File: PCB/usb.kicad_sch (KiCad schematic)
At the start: 52 parts, among them J2 Conn_ARM_SWD_TagConnect_TC2030, J4 TYPE-C-31-M-12, U10 FT2232HQ, U3 TPD2EUSB30, U4 TPD2EUSB30, U6 TPD2EUSB30, U8 TPS62132, U9 M93C56-WMN6TP, Y2 12MHz

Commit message: buttons, more footprints, some other stuff
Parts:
- R29, R32, R36, R37: footprint (none) -> Resistor_SMD:R_0402_1005Metric
- Y2: footprint (none) -> Crystal:Crystal_SMD_3225-4Pin_3.2x2.5mm
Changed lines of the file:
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@@
 			)
 		)
-		(property "Footprint" ""
+		(property "Footprint" "Crystal:Crystal_SMD_3225-4Pin_3.2x2.5mm"
 			(at 125.73 243.84 0)
 			(effects
@@
 			)
 		)
-		(property "Footprint" ""
+		(property "Footprint" "Resistor_SMD:R_0402_1005Metric"
 			(at 293.37 166.878 90)
 			(effects
@@
 			)
 		)
-		(property "Footprint" ""
+		(property "Footprint" "Resistor_SMD:R_0402_1005Metric"
 			(at 293.37 169.418 90)
 			(effects
@@
 			)
 		)
-		(property "Footprint" ""
+		(property "Footprint" "Resistor_SMD:R_0402_1005Metric"
 			(at 293.37 161.798 90)
 			(effects
@@
 			)
 		)
-		(property "Footprint" ""
+		(property "Footprint" "Resistor_SMD:R_0402_1005Metric"
 			(at 293.37 164.338 90)
 			(effects

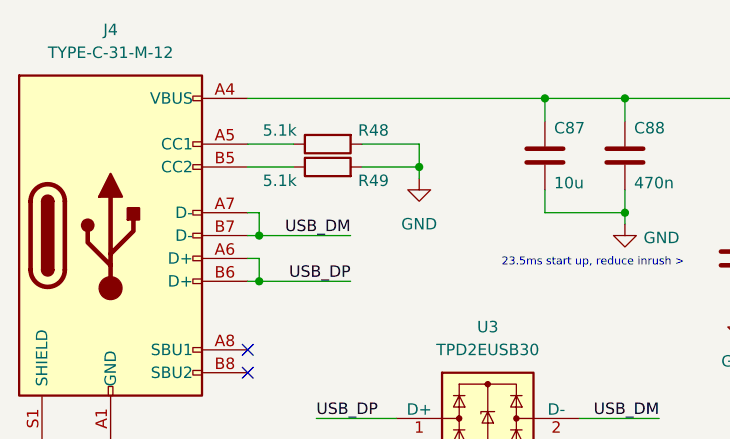
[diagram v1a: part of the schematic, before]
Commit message: adding most of the resistor footprints
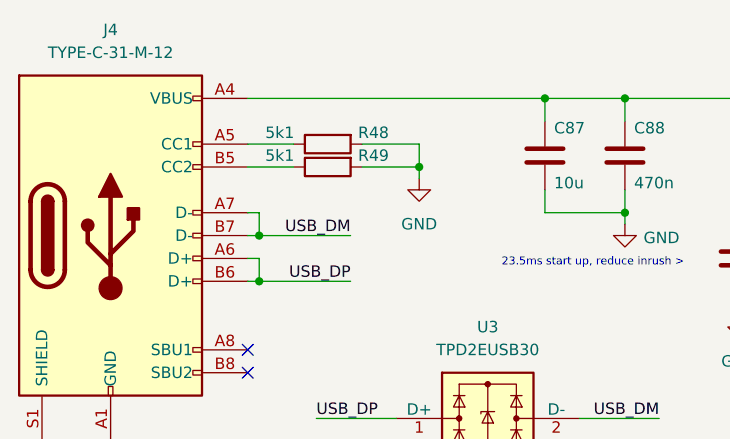
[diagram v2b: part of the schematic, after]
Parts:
- R38, R39, R40, R41, R51, R53, R54: footprint (none) -> Resistor_SMD:R_0402_1005Metric
- R48, R49: value 5.1k -> 5k1
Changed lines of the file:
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@@
 			)
 		)
-		(property "Footprint" ""
+		(property "Footprint" "Resistor_SMD:R_0402_1005Metric"
 			(at 94.742 217.17 90)
 			(effects
@@
 	)
 	(symbol
+		(lib_id "Device:R")
+		(at 59.69 35.56 90)
+		(mirror x)
+		(unit 1)
+		(exclude_from_sim no)
+		(in_bom yes)
+		(on_board yes)
+		(dnp no)
+		(property "Reference" "R49"
+			(at 64.77 34.29 90)
+			(effects
+				(font
+					(size 1.27 1.27)
+				)
+			)
+		)
+		(property "Value" "5k1"
+			(at 54.356 34.29 90)
+			(effects
+				(font
+					(size 1.27 1.27)
+				)
+			)
+		)
+		(property "Footprint" ""
+			(at 59.69 33.782 90)
+			(effects
+				(font
+					(size 1.27 1.27)
+				)
+				(hide yes)
+			)
+		)
+		(property "Datasheet" "~"
+			(at 59.69 35.56 0)
+			(effects
+				(font
+					(size 1.27 1.27)
+				)
+				(hide yes)
+			)
+		)
+		(property "Description" "Resistor"
+			(at 59.69 35.56 0)
+			(effects
+				(font
+					(size 1.27 1.27)
+				)
+				(hide yes)
+			)
+		)
+		(pin "2"
+		)
+		(pin "1"
+		)
+		(instances
+			(project "PCB"
+				(path "/ed0095eb-57a0-4856-9ac4-7b40bd214a3a/b3feae67-f5ac-44a3-90a4-88fd0a4da47c"
+					(reference "R49")
+					(unit 1)
+				)
+			)
+		)
+	)
+	(symbol
 		(lib_id "Device:C")
 		(at 119.38 170.18 0)
@@
 			)
 		)
-		(property "Footprint" ""
+		(property "Footprint" "Resistor_SMD:R_0402_1005Metric"
 			(at 304.292 151.13 90)
 			(effects
@@
 	)
 	(symbol
-		(lib_id "Device:R")
-		(at 59.69 35.56 90)
-		(unit 1)
-		(exclude_from_sim no)
-		(in_bom yes)
-		(on_board yes)
-		(dnp no)
-		(property "Reference" "R49"
-			(at 64.77 37.084 90)
-			(effects
-				(font
-					(size 1.27 1.27)
-				)
-			)
-		)
-		(property "Value" "5.1k"
-			(at 54.356 37.084 90)
-			(effects
-				(font
-					(size 1.27 1.27)
-				)
-			)
-		)
-		(property "Footprint" ""
-			(at 59.69 37.338 90)
-			(effects
-				(font
-					(size 1.27 1.27)
-				)
-				(hide yes)
-			)
-		)
-		(property "Datasheet" "~"
-			(at 59.69 35.56 0)
-			(effects
-				(font
-					(size 1.27 1.27)
-				)
-				(hide yes)
-			)
-		)
-		(property "Description" "Resistor"
-			(at 59.69 35.56 0)
-			(effects
-				(font
-					(size 1.27 1.27)
-				)
-				(hide yes)
-			)
-		)
-		(pin "2"
-		)
-		(pin "1"
-		)
-		(instances
-			(project "PCB"
-				(path "/ed0095eb-57a0-4856-9ac4-7b40bd214a3a/b3feae67-f5ac-44a3-90a4-88fd0a4da47c"
-					(reference "R49")
-					(unit 1)
-				)
-			)
-		)
-	)
-	(symbol
 		(lib_id "Power_Protection:TPD2EUSB30")
 		(at 261.62 204.47 0)
@@
 			)
 		)
-		(property "Footprint" ""
+		(property "Footprint" "Resistor_SMD:R_0402_1005Metric"
 			(at 330.962 151.13 90)
 			(effects
@@
 			)
 		)
-		(property "Footprint" ""
+		(property "Footprint" "Resistor_SMD:R_0402_1005Metric"
 			(at 76.962 217.17 90)
 			(effects
@@
 			)
 		)
-		(property "Footprint" ""
+		(property "Footprint" "Resistor_SMD:R_0402_1005Metric"
 			(at 322.072 151.13 90)
 			(effects
@@
 		(dnp no)
 		(property "Reference" "R48"
-			(at 64.77 31.496 90)
+			(at 64.77 31.75 90)
 			(effects
 				(font
@@
 			)
 		)
-		(property "Value" "5.1k"
-			(at 54.356 31.496 90)
+		(property "Value" "5k1"
+			(at 54.356 31.75 90)
 			(effects
 				(font
@@
 			)
 		)
-		(property "Footprint" ""
+		(property "Footprint" "Resistor_SMD:R_0402_1005Metric"
 			(at 85.852 217.17 90)
 			(effects
@@
 			)
 		)
-		(property "Footprint" ""
+		(property "Footprint" "Resistor_SMD:R_0402_1005Metric"
 			(at 313.182 151.13 90)
 			(effects

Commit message: finisehed upassigning resistor footprints
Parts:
- C89: footprint (none) -> Capacitor_SMD:C_0603_1608Metric
- R48, R49, R50, R52, R55, R56, R76: footprint (none) -> Resistor_SMD:R_0402_1005Metric
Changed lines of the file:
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@@
 			)
 		)
-		(property "Footprint" ""
+		(property "Footprint" "Capacitor_SMD:C_0603_1608Metric"
 			(at 106.3752 49.53 0)
 			(effects
@@
 			)
 		)
-		(property "Footprint" ""
+		(property "Footprint" "Resistor_SMD:R_0402_1005Metric"
 			(at 59.69 33.782 90)
 			(effects
@@
 			)
 		)
-		(property "Footprint" ""
+		(property "Footprint" "Resistor_SMD:R_0402_1005Metric"
 			(at 130.81 199.898 90)
 			(effects
@@
 			)
 		)
-		(property "Footprint" ""
+		(property "Footprint" "Resistor_SMD:R_0402_1005Metric"
 			(at 209.55 240.538 90)
 			(effects
@@
 			)
 		)
-		(property "Footprint" ""
+		(property "Footprint" "Resistor_SMD:R_0402_1005Metric"
 			(at 130.81 194.818 90)
 			(effects
@@
 			)
 		)
-		(property "Footprint" ""
+		(property "Footprint" "Resistor_SMD:R_0402_1005Metric"
 			(at 59.69 31.242 90)
 			(effects
@@
 			)
 		)
-		(property "Footprint" ""
+		(property "Footprint" "Resistor_SMD:R_0402_1005Metric"
 			(at 153.162 41.91 90)
 			(effects
@@
 			)
 		)
-		(property "Footprint" ""
+		(property "Footprint" "Resistor_SMD:R_0402_1005Metric"
 			(at 85.09 235.458 90)
 			(effects
